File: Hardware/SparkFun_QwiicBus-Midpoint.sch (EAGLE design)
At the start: 41 parts, among them J1 QWIIC, J2 QWIIC, J3 RJ45, J7 RJ45, U1 PCA9615, U2 AP63203

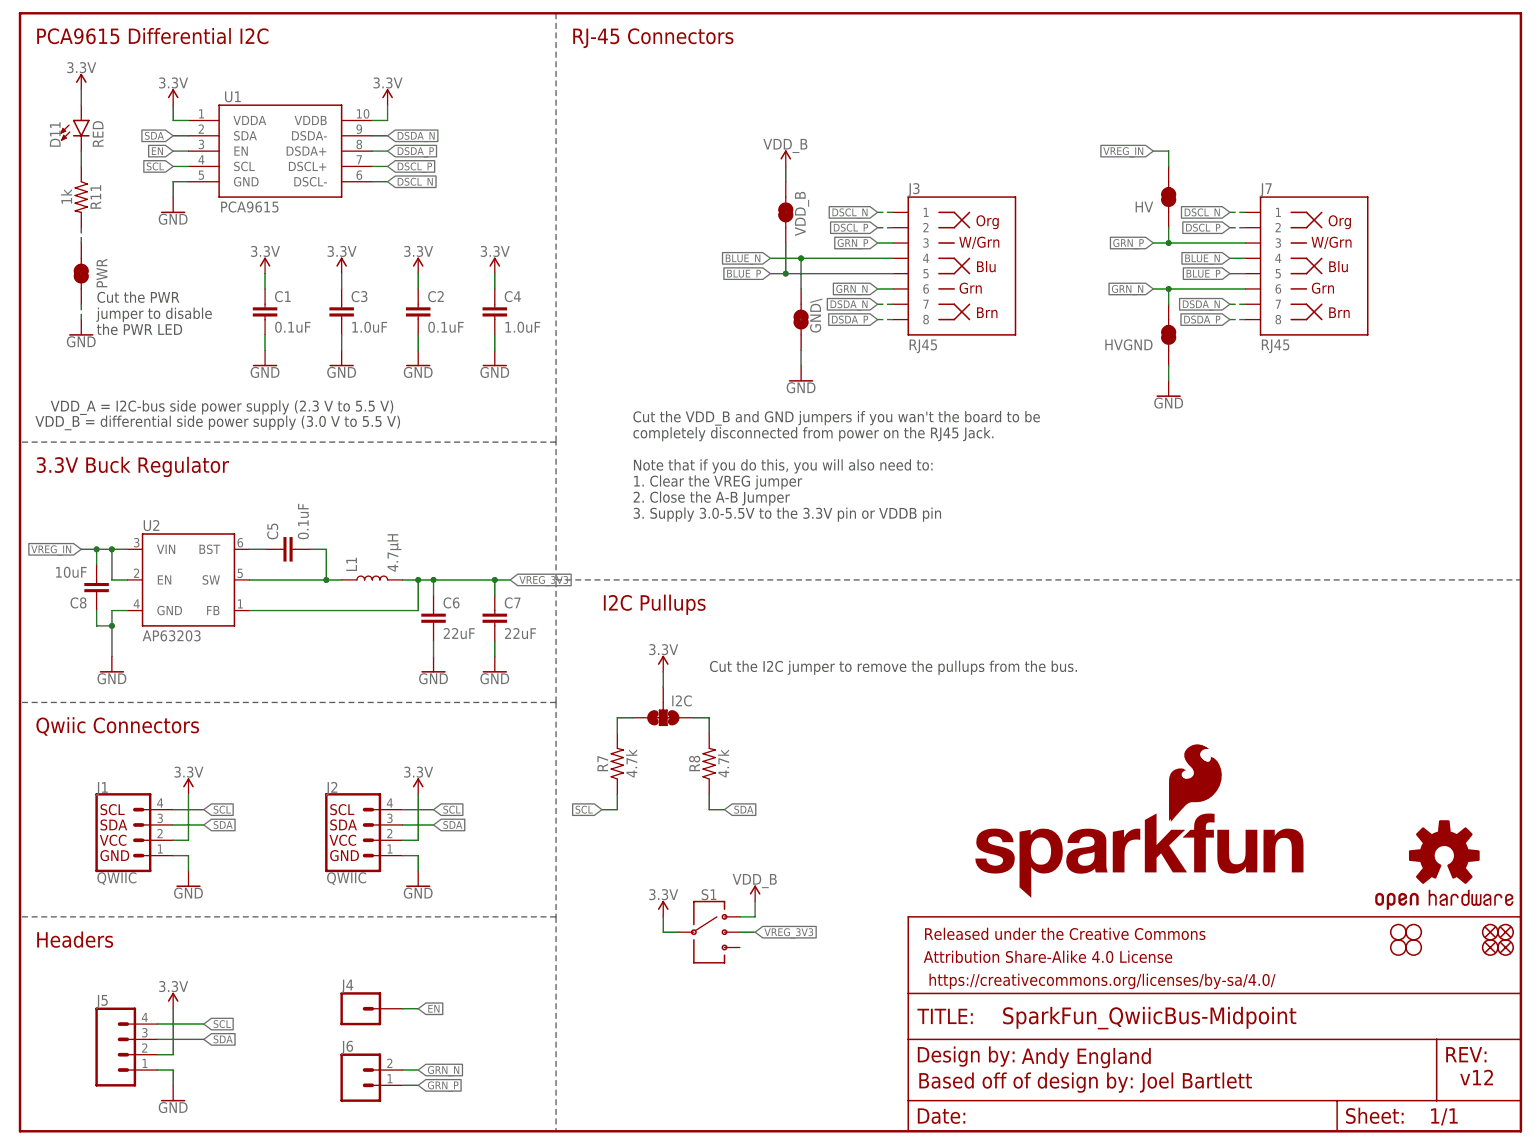
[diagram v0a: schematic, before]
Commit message: post review changes
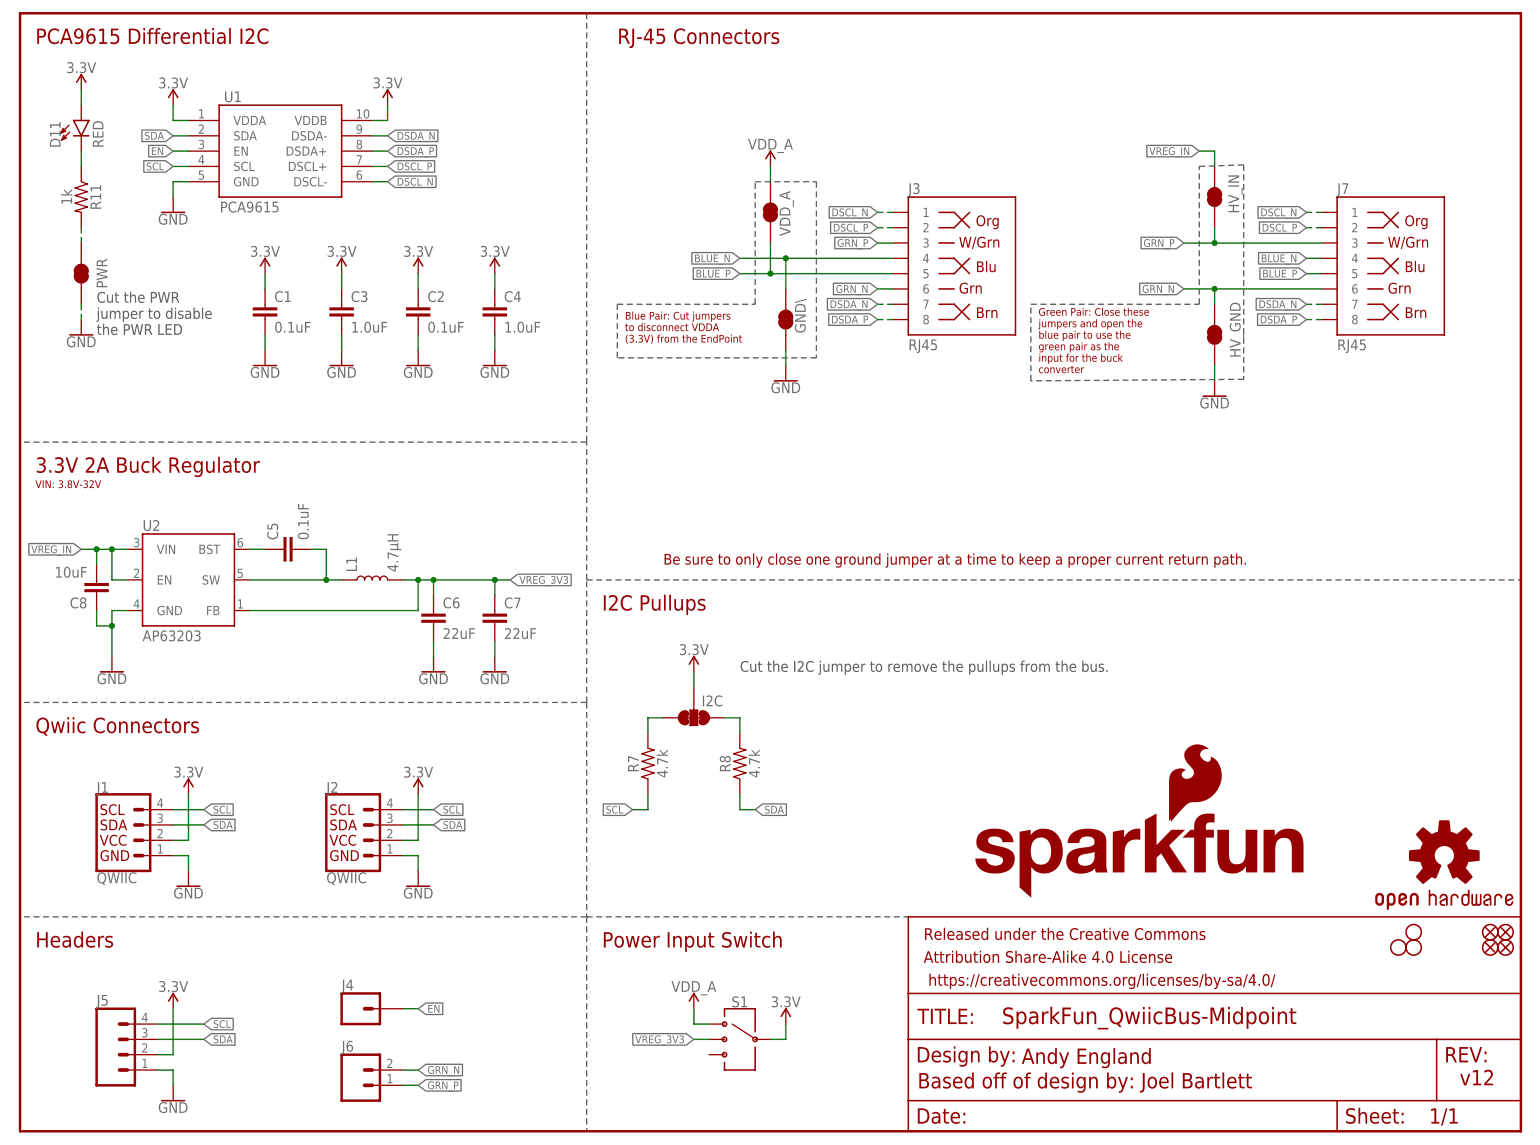
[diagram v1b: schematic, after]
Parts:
- removed H1: STAND-OFF, SparkFun-Hardware:STAND-OFF
- removed HV, HVGND, VDD_B: JUMPER-SMT_2_NC_TRACE_SILK, SparkFun-Jumpers:JUMPER-SMT_2_NC_TRACE_SILK
- added HV_GND, HV_IN, VDD_A: JUMPER-SMT_2_NC_TRACE_SILK, SparkFun-Jumpers:JUMPER-SMT_2_NC_TRACE_SILK
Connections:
- removed net VDD_B: S1.1, VDD_B.1
- new net VDD_A: S1.1, VDD_A.1
- net BLUE_P: now also VDD_A.2; no longer VDD_B.2
- net GND: now also HV_GND.1; no longer HVGND.1
- net GRN_N: now also HV_GND.2; no longer HVGND.2
- net GRN_P: now also HV_IN.1; no longer HV.1
- net VREG_IN: now also HV_IN.2; no longer HV.2
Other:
- note added: "3.3V 2A Buck Regulator"
- note added: "Be sure to only close one ground jumper at a time to keep a proper current return path."
- note added: "Blue Pair: Cut jumpers to disconnect VDDA (3.3V) from the EndPoint"
- note added: "Green Pair: Close these jumpers and open the blue pair to use the green pair as the input for the buck converter"
- note added: "Power Input Switch"
- note added: "VIN: 3.8V-32V"
- note removed: "3.3V Buck Regulator"
- note removed: "Cut the VDD_B and GND jumpers if you wan't the board to be completely disconnected from power on the RJ45 Jack. Note that if you do this, you will also need to: 1. Clear the VREG jumper 2. Close the A-B Jumper 3. Supply 3.0-5.5V to the 3.3V pin or VDDB pin"
- note removed: "VDD_A = I2C-bus side power supply (2.3 V to 5.5 V)"
- note removed: "VDD_B = differential side power supply (3.0 V to 5.5 V)"
- moved on the sheet: GND\, I2C, J7, R7, R8, S1

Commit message: ordering protos
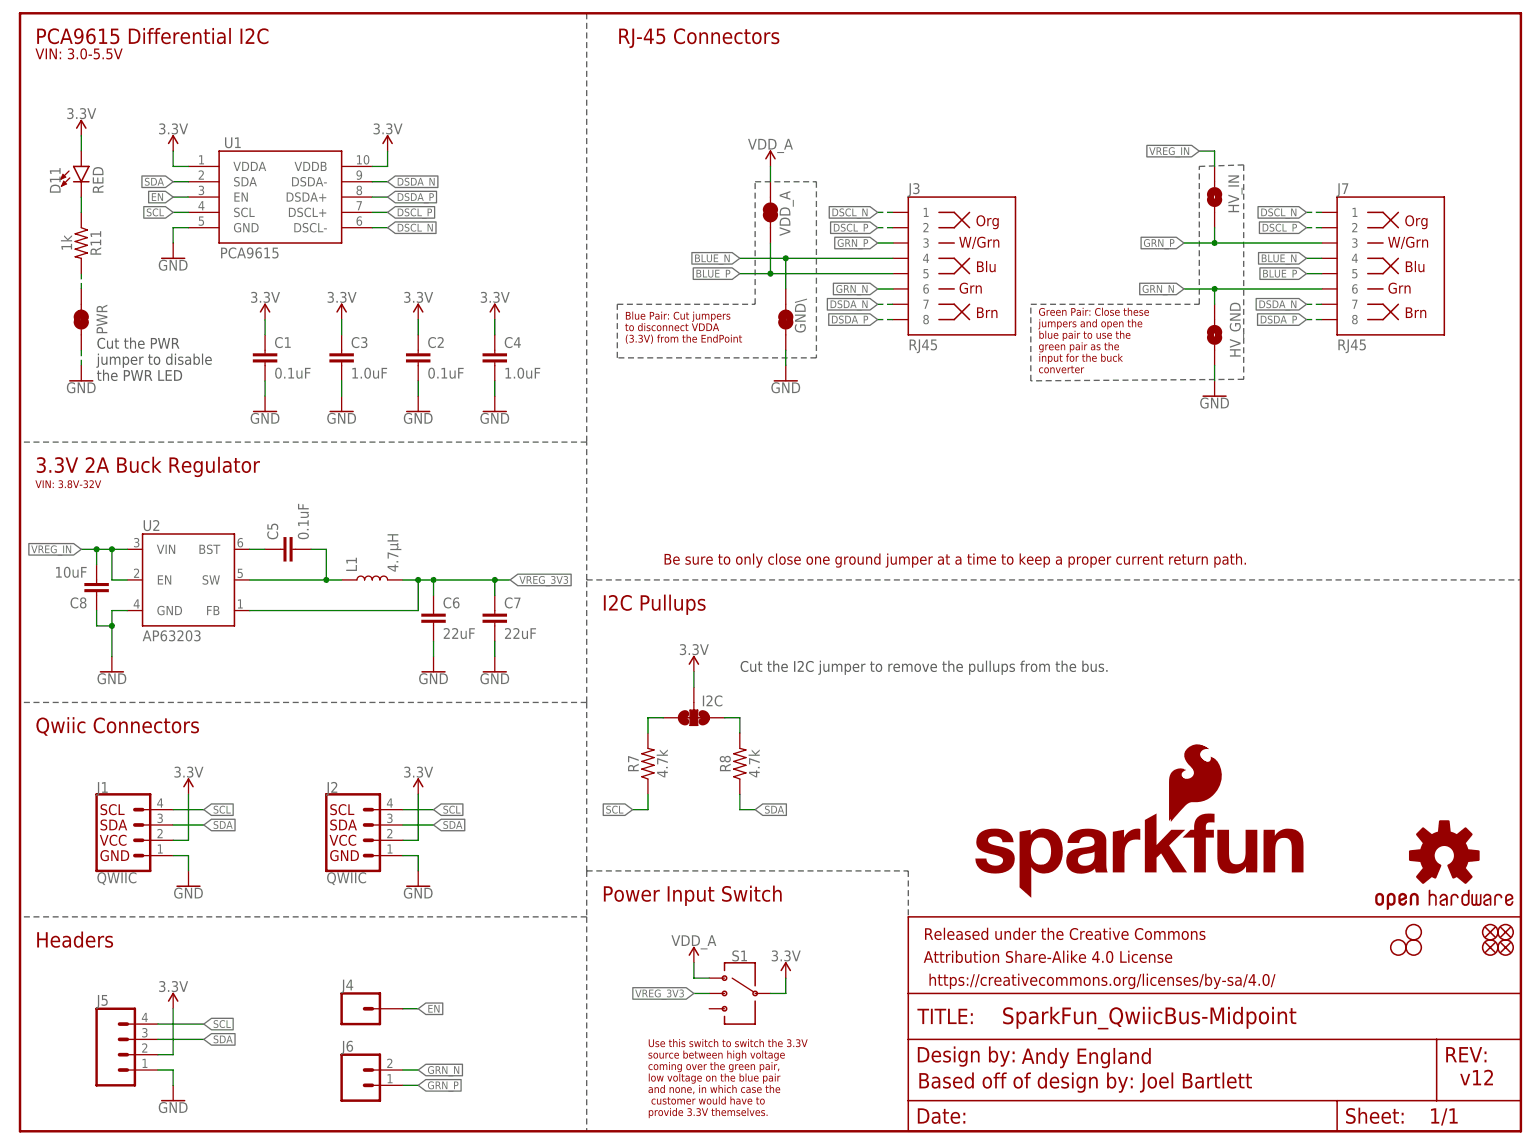
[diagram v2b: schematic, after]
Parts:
- HV_GND, HV_IN: value JUMPER-SMT_2_NC_TRACE_SILK -> JUMPER-SMT_2_NO_SILK; device SparkFun-Jumpers:JUMPER-SMT_2_NC_TRACE_SILK -> SparkFun-Jumpers:JUMPER-SMT_2_NO_SILK
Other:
- note added: "Use this switch to switch the 3.3V source between high voltage coming over the green pair, low voltage on the blue pair and none, in which case the customer would have to provide 3.3V themselves."
- note added: "VIN: 3.0-5.5V"
- moved on the sheet: C1, C2, C3, C4, D11, PWR, R11, S1, U1

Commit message: post FarmHand Review
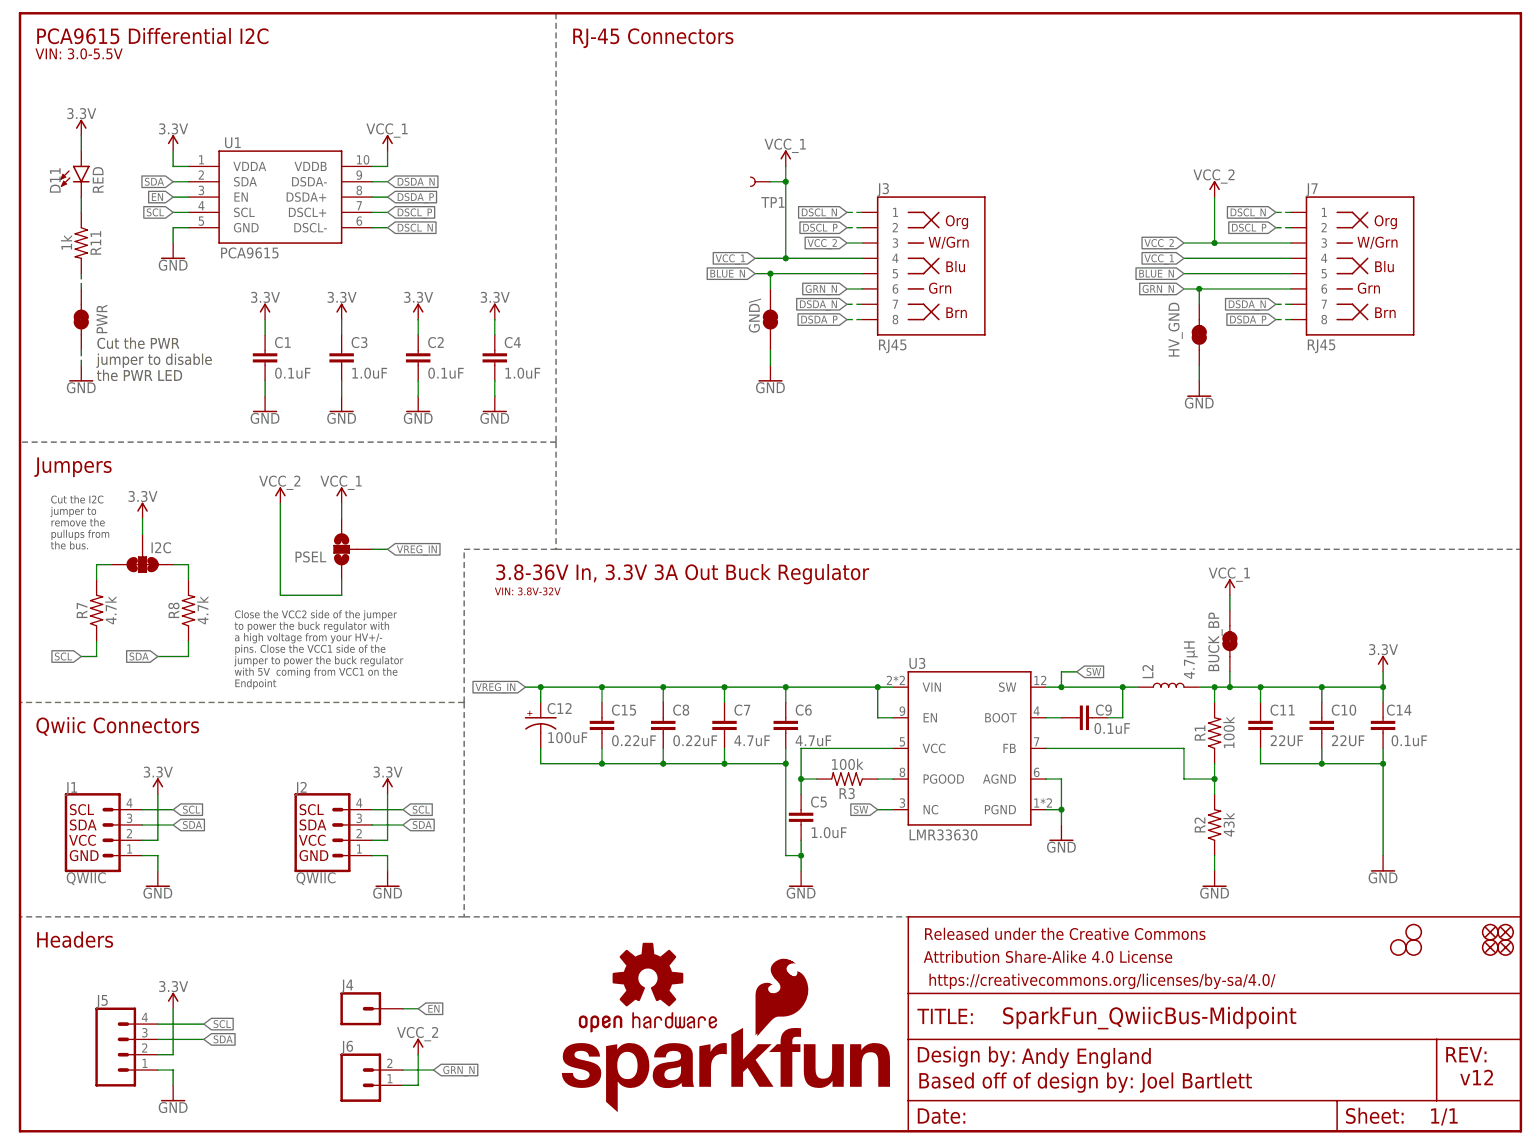
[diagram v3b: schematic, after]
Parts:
- removed HV_IN: JUMPER-SMT_2_NO_SILK, SparkFun-Jumpers:JUMPER-SMT_2_NO_SILK
- removed L1: 4.7μH, SparkFun-Coils:4.7μH_SHIELDED_INDUCTORNPIS_LS
- removed S1: (no value), SparkFun-Switches:SWITCH-SP3T-SMD
- removed U2: AP63203, SparkFun-IC-Power:AP63203
- removed VDD_A: JUMPER-SMT_2_NC_TRACE_SILK, SparkFun-Jumpers:JUMPER-SMT_2_NC_TRACE_SILK
- added BUCK_BP: JUMPER-SMT_2_NC_TRACE_SILK, SparkFun-Jumpers:JUMPER-SMT_2_NC_TRACE_SILK
- added C10, C11: 22UF, SparkFun-Capacitors:22UF-1210-16V-20%
- added C12: 100uF, SparkFun-Capacitors:100UF-POLAR-8X10.5-50V
- added C14, C9: 0.1uF, SparkFun-Capacitors:0.1UF-0603-100V-10%
- added C15: 0.22uF, SparkFun-Capacitors:0.22UF-0603-25V-10%
- added L2: 4.7μH, SparkFun-Coils:4.7μH_SHIELDED_INDUCTORNPIS_LS
- added PSEL: JUMPER-SMT_3_NO_SILK, SparkFun-Jumpers:JUMPER-SMT_3_NO_SILK
- added R1, R3: 100k, SparkFun-Resistors:100KOHM-0603-1/10W-1%
- added R2: 43k, SparkFun-Resistors:43KOHM-0603-1/10W-1%
- added TP1: TEST-POINT3, SparkFun-Connectors:TEST-POINT3
- added U3: LMR33630, SparkFun-IC-Power:LMR33630
- C5: value 0.1uF -> 1.0uF; device SparkFun-Capacitors:0.1UF-0603-100V-10% -> SparkFun-Capacitors:1.0UF-0603-16V-10%
- C6, C7: value 22uF -> 4.7uF; device SparkFun-Capacitors:22UF-1206-50V-10% -> SparkFun-Capacitors:4.7UF-0805-50V-(10%)
- C8: value 10uF -> 0.22uF; device SparkFun-Capacitors:10UF-1210-50V-20% -> SparkFun-Capacitors:0.22UF-0603-25V-10%
- HV_GND: value JUMPER-SMT_2_NO_SILK -> JUMPER-SMT_2_NC_TRACE_SILK; device SparkFun-Jumpers:JUMPER-SMT_2_NO_SILK -> SparkFun-Jumpers:JUMPER-SMT_2_NC_TRACE_SILK
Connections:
- removed net BLUE_P: J3.5, J7.5, VDD_A.2
- removed net GRN_P: HV_IN.1, J3.3, J6.1, J7.3
- removed net N$8: C5.2, L1.1, U2.SW
- removed net VDD_A: S1.1, VDD_A.1
- removed net VREG_3V3: C6.1, C7.1, L1.2, S1.2, U2.FB
- new net N$1: C9.1, U3.BOOT
- new net N$6: R1.1, R2.2, U3.FB
- new net N$9: C5.1, R3.2, U3.VCC
- new net SW: C9.2, L2.1, U3.NC, U3.SW
- new net VCC_1: BUCK_BP.2, J3.4, J7.4, PSEL.3, TP1.1, U1.VDDB
- new net VCC_2: J3.3, J6.1, J7.3, PSEL.1
- net 3.3V: now also BUCK_BP.1, C10.1, C11.1, C14.1, L2.2, R1.2; no longer S1.3, U1.VDDB
- net BLUE_N: now also J3.5, J7.5; no longer J3.4, J7.4
- net GND: now also C10.2, C11.2, C12.-, C14.2, C15.2, C5.2, C8.2, R2.1, U3.AGND, U3.PGND; no longer C8.1, U2.GND
- net N$7: now also R3.1, U3.PGOOD; no longer C5.1, U2.BST
- net VREG_IN: now also C12.+, C15.1, C6.1, C7.1, C8.1, PSEL.2, U3.EN, U3.VIN; no longer C8.2, HV_IN.2, U2.EN, U2.VIN
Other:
- note added: "3.8-36V In, 3.3V 3A Out Buck Regulator"
- note added: "Close the VCC2 side of the jumper to power the buck regulator with a high voltage from your HV+/- pins. Close the VCC1 side of the jumper to power the buck regulator with 5V coming from VCC1 on the Endpoint"
- note added: "Jumpers"
- note removed: "3.3V 2A Buck Regulator"
- note removed: "Be sure to only close one ground jumper at a time to keep a proper current return path."
- note removed: "Blue Pair: Cut jumpers to disconnect VDDA (3.3V) from the EndPoint"
- note removed: "Green Pair: Close these jumpers and open the blue pair to use the green pair as the input for the buck converter"
- note removed: "I2C Pullups"
- note removed: "Power Input Switch"
- note removed: "Use this switch to switch the 3.3V source between high voltage coming over the green pair, low voltage on the blue pair and none, in which case the customer would have to provide 3.3V themselves."
- moved on the sheet: C5, C6, C7, C8, GND\, I2C, J1, J2, J3, J7, R7, R8
